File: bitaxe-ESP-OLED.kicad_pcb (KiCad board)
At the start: 2 copper layers, 57.4 x 42 mm, 48 parts, among them J1 SFV30R-4STE1HLF, J2 Conn_01x06, J3 USB_C_Receptacle_USB2.0_16P, Q1 SI2307, SW1 SWITCH-SPST, SW2 SWITCH-SPST, SW3 SWITCH-SPST, SW4 SWITCH-SPST, U1 ESP32_S3R8, U2 RT9080-33GJ5, U3 AP2502KTR-G1, U4 W25Q128JV

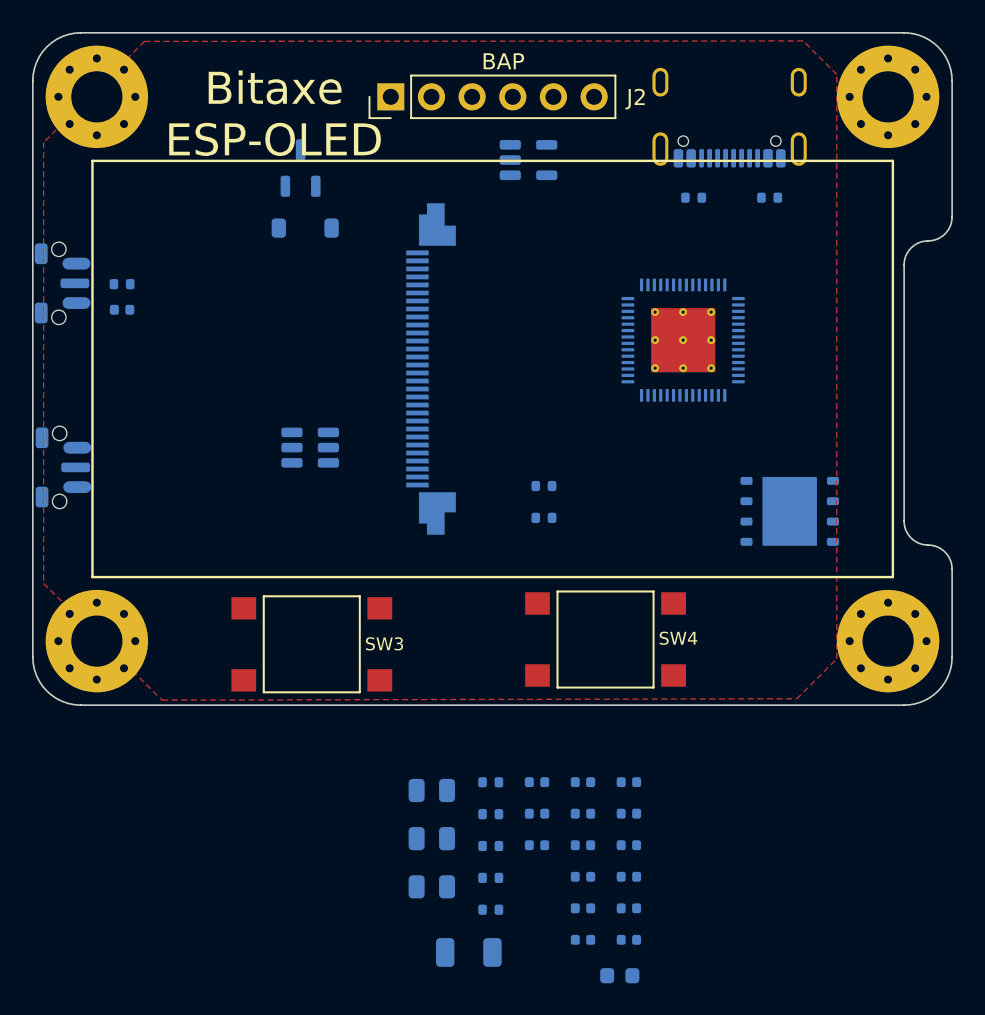
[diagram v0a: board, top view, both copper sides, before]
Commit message: very rough routing
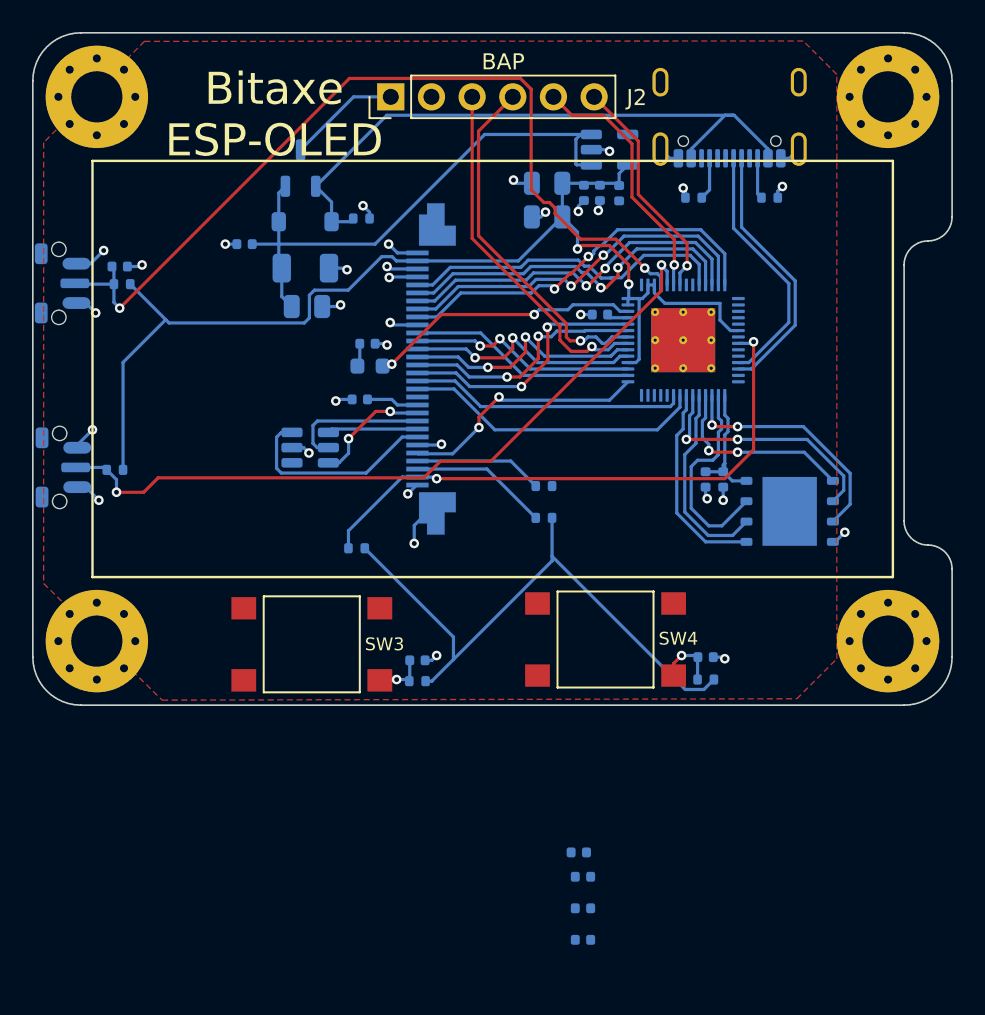
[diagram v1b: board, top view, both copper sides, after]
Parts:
- moved C2 44.0 mm to (146.6, 76.7), turned to 0 degrees
- moved C21 42.5 mm to (161.7, 73.5)
- moved C13 41.6 mm to (161.7, 71.4)
- moved C3 41.3 mm to (142.8, 75.2)
- moved L1 41.2 mm to (150.6, 82.8), turned to 0 degrees
- moved C19 41.1 mm to (166.2, 72.0), turned to -90 degrees
- moved C18 39.0 mm to (165.0, 72.0), turned to 90 degrees
- moved C17 36.9 mm to (164.0, 72.0), turned to -90 degrees
- moved R1 36.1 mm to (150.1, 73.6), turned to 0 degrees
- moved C11 32.3 mm to (150.5, 81.4)
- moved R5 31.8 mm to (134.7, 89.3)
- moved C1 31.2 mm to (146.7, 79.1), turned to 0 degrees
- moved C4 30.9 mm to (150.0, 84.9), turned to 0 degrees
- moved C10 29.2 mm to (165.0, 79.6), turned to 0 degrees
- moved C9 29.2 mm to (171.6, 89.9), turned to -90 degrees
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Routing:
- net /3V3: track 0.00 -> 109.2 mm, vias 0 -> 2
- net /RESET: track 0.00 -> 54.5 mm, vias 0 -> 2
- net /GPIO0: track 0.00 -> 45.9 mm, vias 0 -> 2
- net GND: track 0.00 -> 41.3 mm, vias 0 -> 32
- net /VBUS: track 0.00 -> 39.6 mm
- net /TP_INT: track 0.00 -> 36.3 mm, vias 0 -> 2
- net /+5V: track 0.00 -> 35.7 mm
- net /LCD_RD: track 0.00 -> 24.3 mm, vias 0 -> 2
- net /LCD_WR: track 0.00 -> 23.3 mm, vias 0 -> 2
- net /LCD_DC: track 0.00 -> 22.7 mm, vias 0 -> 2
- net /BAP_RX: track 0.00 -> 22.5 mm, vias 0 -> 1
- net /BAP_TX: track 0.00 -> 22.4 mm, vias 0 -> 1
- net /LCD_CS: track 0.00 -> 22.3 mm, vias 0 -> 2
- net /LCD_RES: track 0.00 -> 20.8 mm
- net /LCD_D7: track 0.00 -> 18.8 mm
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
